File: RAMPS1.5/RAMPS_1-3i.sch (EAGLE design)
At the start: 96 parts, among them SW1 SPST_TACT-EVQQ2, U1 ARDUINO_MEGA_SHIELD

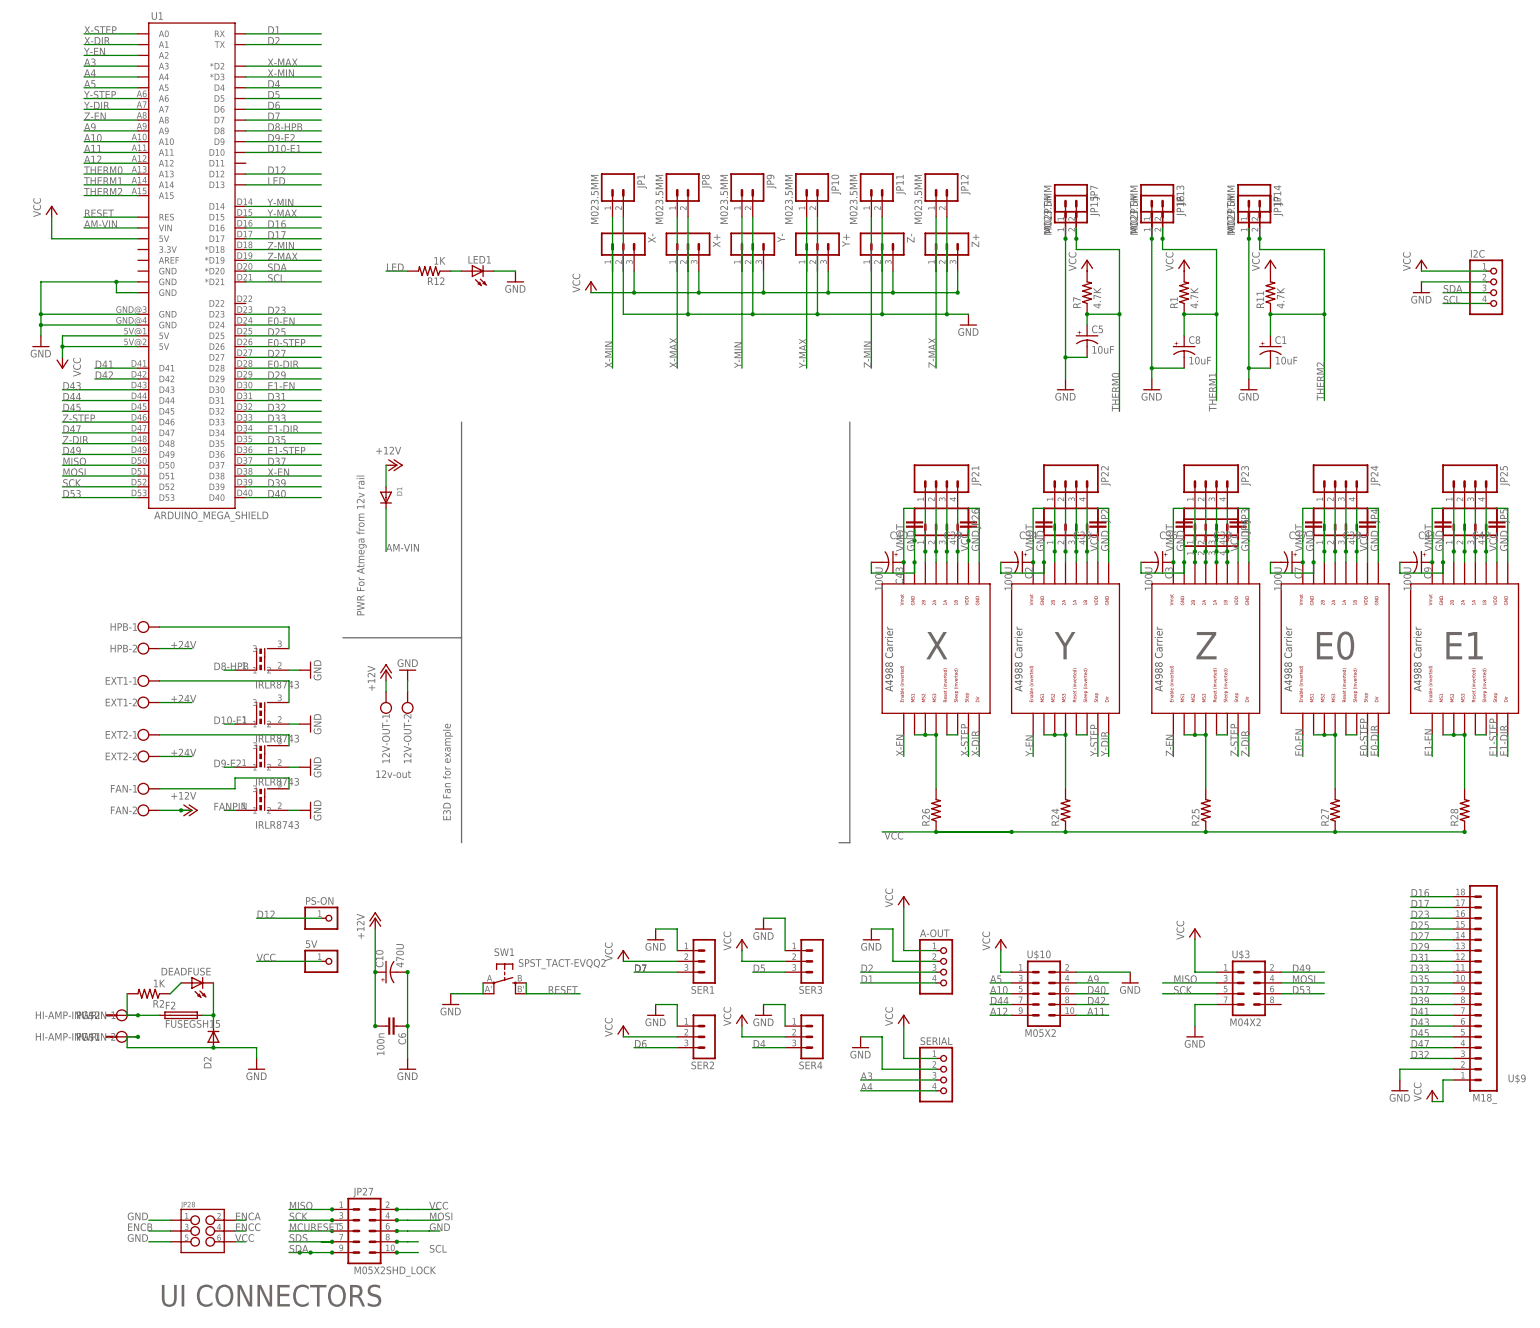
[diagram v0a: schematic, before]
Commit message: HY28 and Ramps1.5
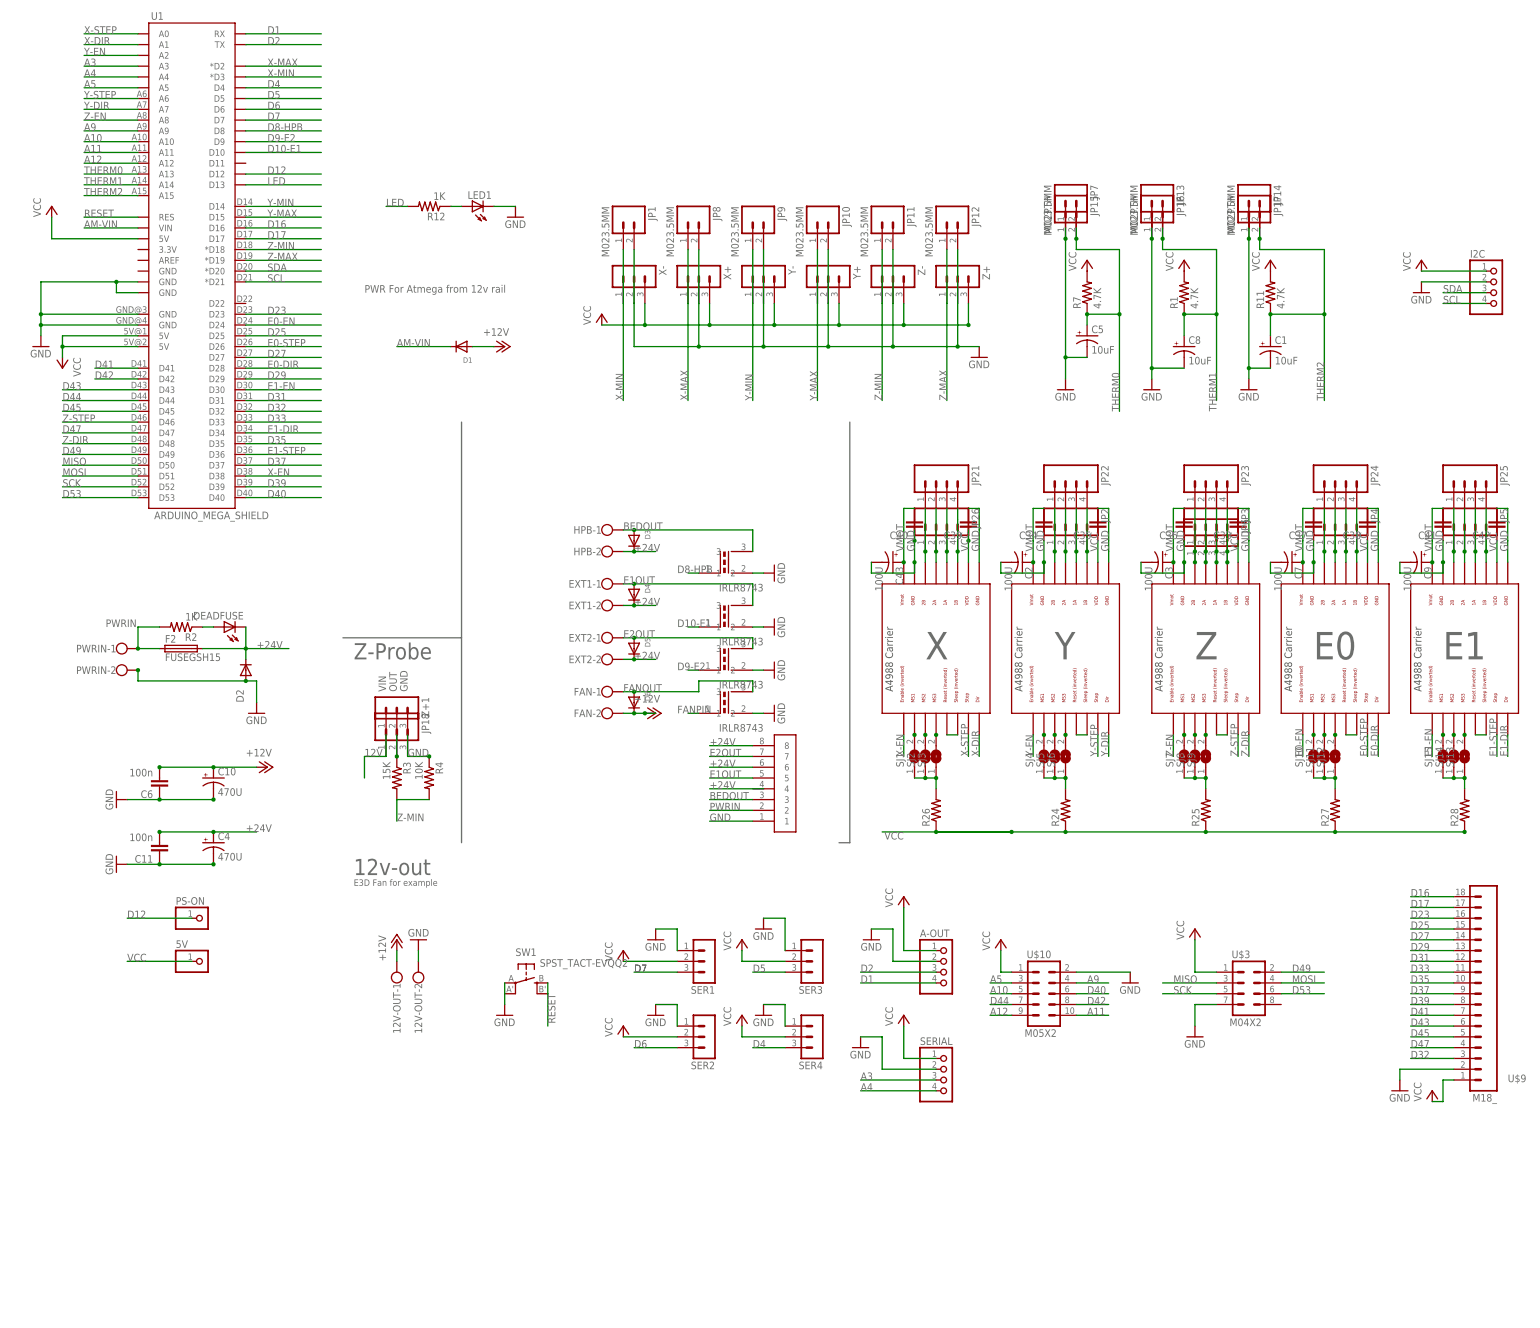
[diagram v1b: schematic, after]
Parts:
- removed HI-AMP-IN: DEGSON_2, Simplex-Connectors:DEGSON_2
- removed JP27: M05X2SHD_LOCK, SparkFun-Connectors:M05X2SHD_LOCK
- removed JP28: (no value), SparkFun-Connectors:M03X2SHROUD
- added C11: 100n, SparkFun-Passives:CAP1206
- added C4: 470U, SparkFun-Capacitors:CAP_POLD
- added D3, D4, D5, D6: (no value), adafruit:DIODESMA
- added JP18: (no value), SparkFun-Connectors:M03SCREW_LOCK
- added R3: 15K, adafruit:R-US_M1206
- added R4: 10K, adafruit:R-US_M1206
- added SJ1, SJ10, SJ11, SJ12, SJ13, SJ14, SJ15, SJ2, SJ3, SJ4, SJ5, SJ6, SJ7, SJ8, SJ9: (no value), jumper:SJ
- added U$4: XY825A-8P, Communica.co.za:XY825A-8P
- added Z+1: (no value), ultimachine:3PIN-HEADER
- R12: device adafruit:R-US_0207/7 -> adafruit:R-US_M1206
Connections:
- removed net ENCA: JP28.2
- removed net ENCB: JP28.3
- removed net ENCC: JP28.4
- removed net MCURESET: JP27.5
- removed net N$1: EXT2-1.KL, U$11.3
- removed net N$2: HPB-1.KL, U$2.3
- removed net N$32: F2.1, HI-AMP-ING$2.KL, PWRIN-1.KL, R2.2
- removed net N$47: EXT1-1.KL, U$12.3
- removed net N$5: FAN-1.KL, U$1.3
- removed net N$66: JP27.8
- removed net SDS: JP27.7
- new net 12V: JP18.1, Z+1.1
- new net BEDOUT: D3.A, HPB-1.KL, U$2.3, U$4.3
- new net E1OUT: D4.A, EXT1-1.KL, U$12.3, U$4.5
- new net E2OUT: D5.A, EXT2-1.KL, U$11.3, U$4.7
- new net FANOUT: D6.A, FAN-1.KL, U$1.3
- new net N$10: SJ8.2, ZPOL1.MS2
- new net N$11: SJ9.2, ZPOL1.MS3
- new net N$12: SJ6.2, YPOL1.MS3
- new net N$13: SJ3.2, XPOL1.MS3
- new net N$14: E2POL1.MS2, SJ14.2
- new net N$15: E2POL1.MS3, SJ13.2
- new net N$16: E2POL1.MS1, SJ15.2
- new net N$17: E1POL1.MS3, SJ12.2
- new net N$18: E1POL1.MS1, SJ10.2
- new net N$19: E1POL1.MS2, SJ11.2
- new net N$6: SJ1.2, XPOL1.MS1
- new net N$7: SJ4.2, YPOL1.MS1
- new net N$8: SJ5.2, YPOL1.MS2
- new net N$9: SJ7.2, ZPOL1.MS1
- new net PWRIN: F2.1, PWRIN-1.KL, R2.2, U$4.2
- new net SENSOROUT: JP18.2, R3.1, Z+1.2
- net +12V: now also D6.C
- net +24V: now also C11.2, C4.+, D2.C, D3.C, D4.C, D5.C, DEADFUSE.C, F2.2, U$4.6, U$4.8
- net GND: now also C11.1, C4.-, JP18.3, R4.1, U$4.1, Z+1.3; no longer HI-AMP-ING$1.KL, JP27.6, JP28.1, JP28.5
- net MISO: no longer JP27.1
- net MOSI: no longer JP27.4
- net N$4: now also SJ2.2, XPOL1.MS2; no longer D2.C, DEADFUSE.C, F2.2
- net N$58: now also SJ1.1, SJ2.1, SJ3.1; no longer XPOL1.MS1, XPOL1.MS2, XPOL1.MS3
- net N$59: now also SJ4.1, SJ5.1, SJ6.1; no longer YPOL1.MS1, YPOL1.MS2, YPOL1.MS3
- net N$60: now also SJ10.1, SJ11.1, SJ12.1; no longer E1POL1.MS1, E1POL1.MS2, E1POL1.MS3
- net N$62: now also SJ7.1, SJ8.1, SJ9.1; no longer ZPOL1.MS1, ZPOL1.MS2, ZPOL1.MS3
- net N$84: now also SJ13.1, SJ14.1, SJ15.1; no longer E2POL1.MS1, E2POL1.MS2, E2POL1.MS3
- net SCK: no longer JP27.3
- net SCL: no longer JP27.10
- net SDA: no longer JP27.9
- net VCC: no longer JP27.2, JP28.6
- net Z-MIN: now also R3.2, R4.2
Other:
- note added: "GND"
- note added: "OUT"
- note added: "VIN"
- note added: "Z-Probe"
- note removed: "UI CONNECTORS"
- moved on the sheet: 12V-OUT-1, 12V-OUT-2, 5V, C10, C6, D1, D2, DEADFUSE, EXT1-1, EXT1-2, EXT2-1, EXT2-2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
